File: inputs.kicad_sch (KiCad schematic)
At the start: 62 parts, among them J4 TPS43, SW1 KEY_A, SW10 D2F-01F, SW11 D2F-01F, SW12 D2F-01F, SW13 RKB2SJM250SMTR, SW14 RKB2SJM250SMTR, SW15 RKB2SJM250SMTR, SW2 KEY_B, SW3 KEY_C, SW4 KEY_D, SW5 KEY_E, SW6 KEY_F, SW7 D2F-01F, SW8 D2F-01F, SW9 D2F-01F

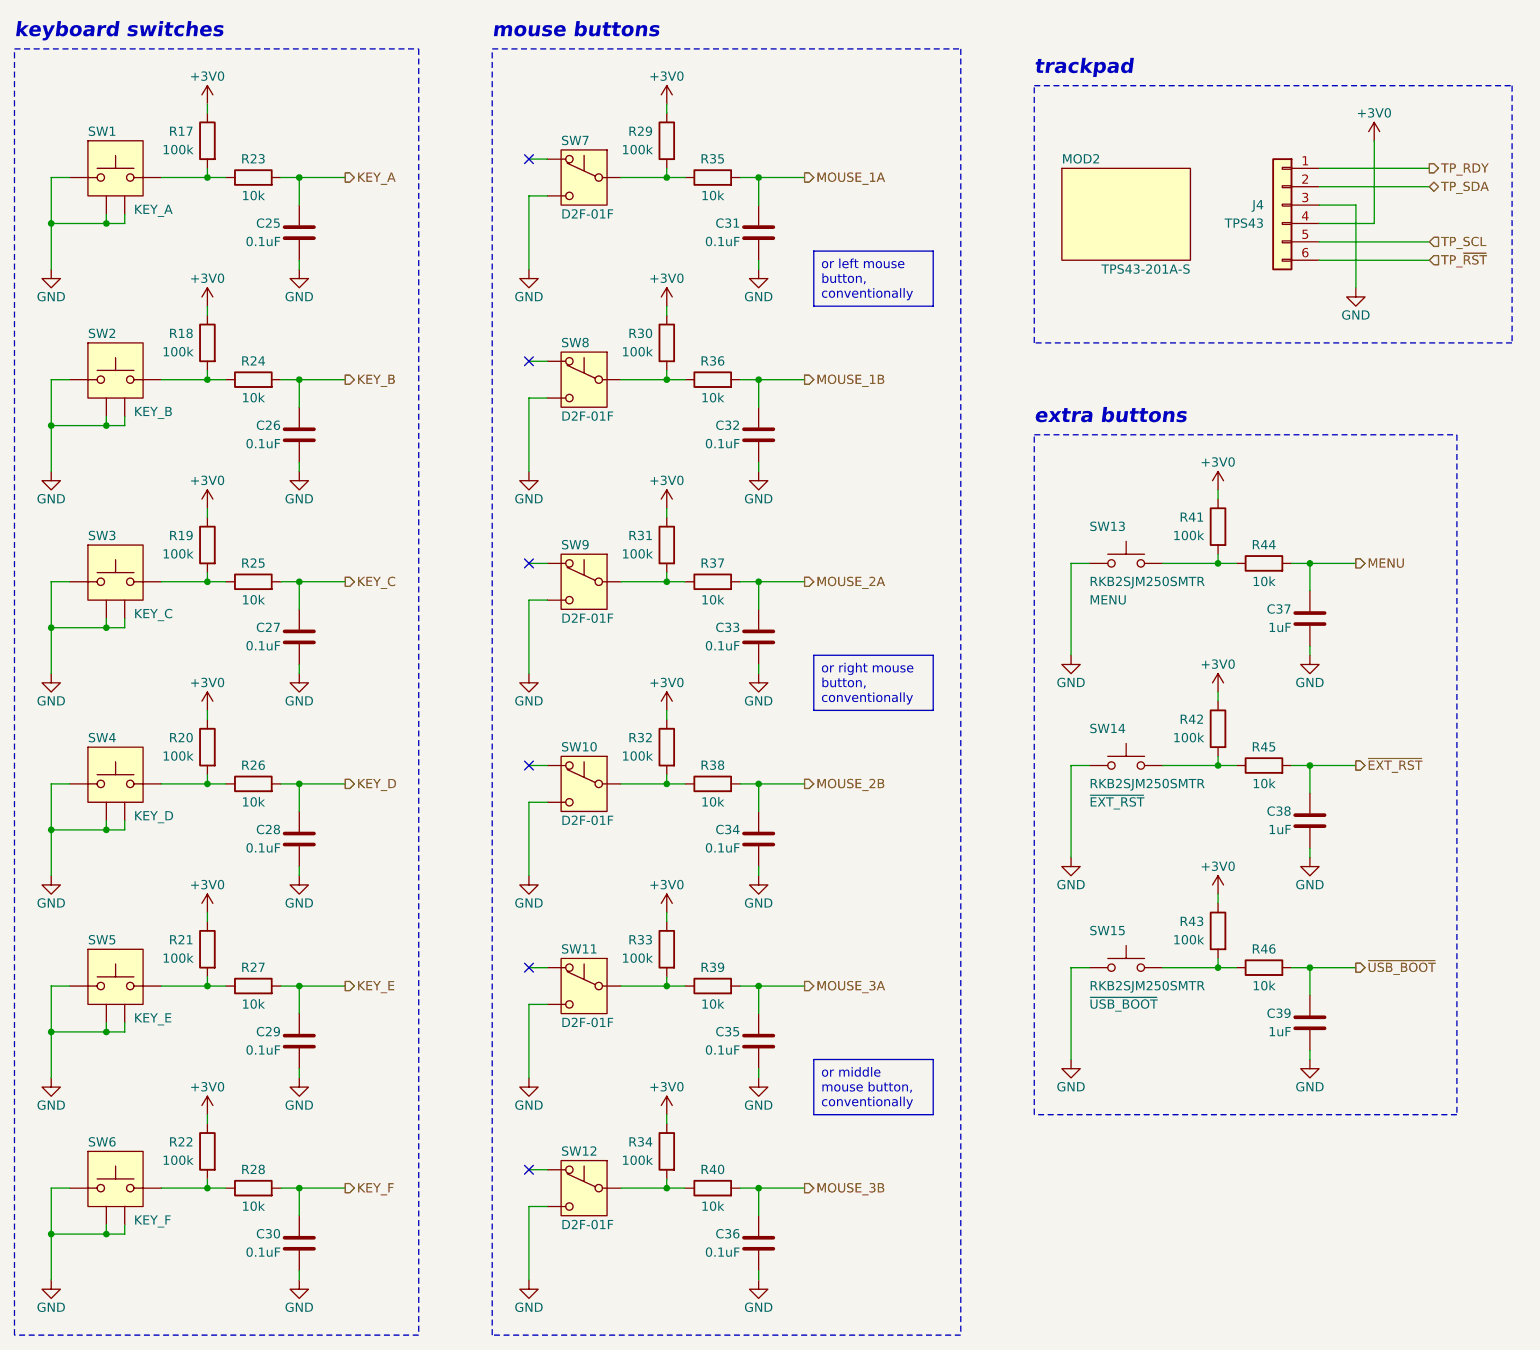
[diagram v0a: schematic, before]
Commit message: new mouse button setup
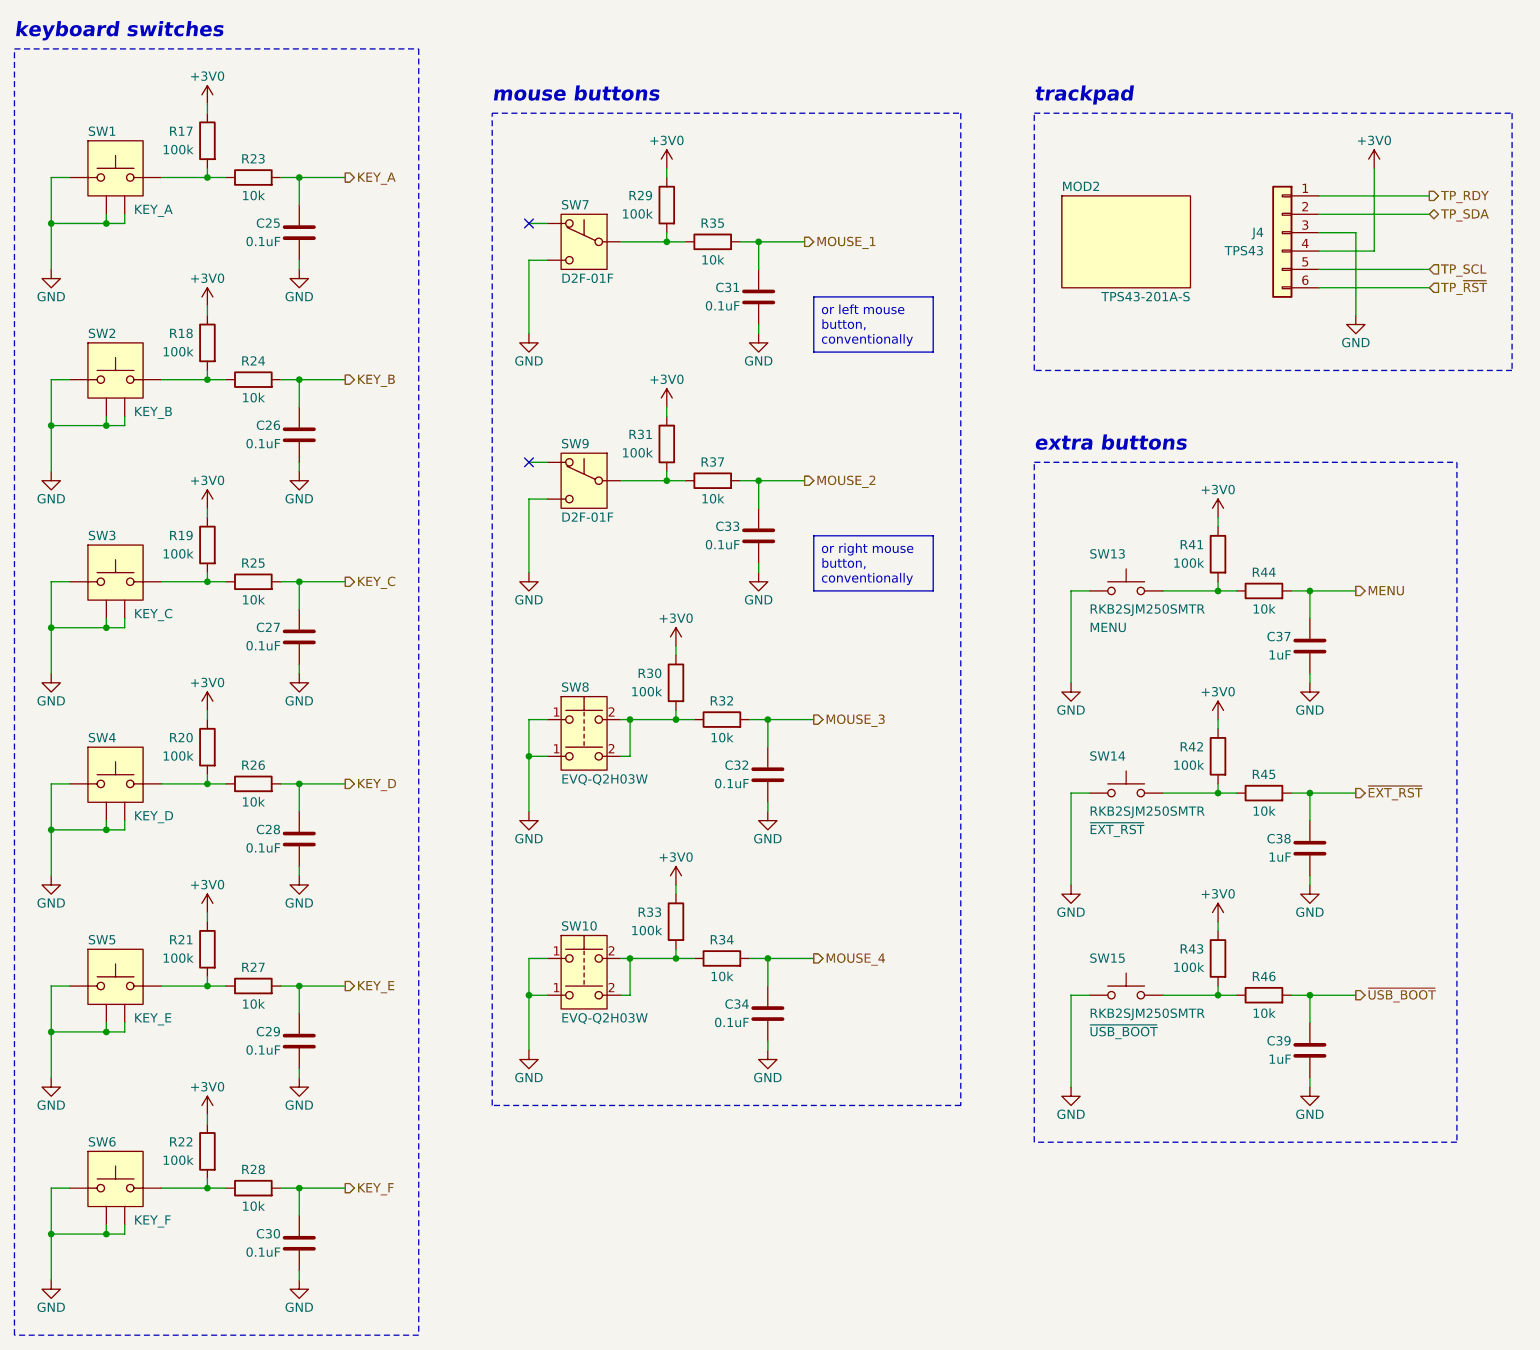
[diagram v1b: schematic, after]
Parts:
- removed C35, C36: 0.1uF, Capacitor_SMD:C_0805_2012Metric, symbol Device:C
- removed R36, R38, R39, R40: 10k, Resistor_SMD:R_0805_2012Metric, symbol Device:R
- removed SW10, SW11, SW12, SW8: D2F-01F, footprints:D2F01F, symbol user:D2F-01F
- added SW10, SW8: EVQ-Q2H03W, footprints:EVQ-Q2H03W, symbol Switch:SW_Push_Dual
- R32, R34: value 100k -> 10k
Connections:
- net MOUSE_1B is gone; now on net MOUSE_3: C32.1
- net MOUSE_2B is gone; now on net MOUSE_4: C34.1
- net +3V0: no longer R32.1, R34.1
- net GND: now also SW10.1 (1b), SW8.1 (1b)
- net MOUSE_4: now reaches R34.2
- net at R33.2: now also R34.1, SW10.2 (2b)
- net MOUSE_3: now reaches R32.2
- net at R30.2: now also R32.1, SW8.2 (2b)
- net MOUSE_1A renamed MOUSE_1
- net MOUSE_2A renamed MOUSE_2
- no-connect marks 6 -> 2
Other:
- moved on the sheet: C31, C33, C37, C38, C39, J4, MOD2, R29, R31, R35, R37, R41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
